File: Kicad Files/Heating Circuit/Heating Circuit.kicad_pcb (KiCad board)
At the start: 2 copper layers, 73 x 78 mm, 12 parts, among them J1 XT60_F_16.6V, J2 XT60_F_Heater, J3 XT60_F_Thermocouple, Q1 BUK9M52-40EX, U1 MAX31855KASA+T

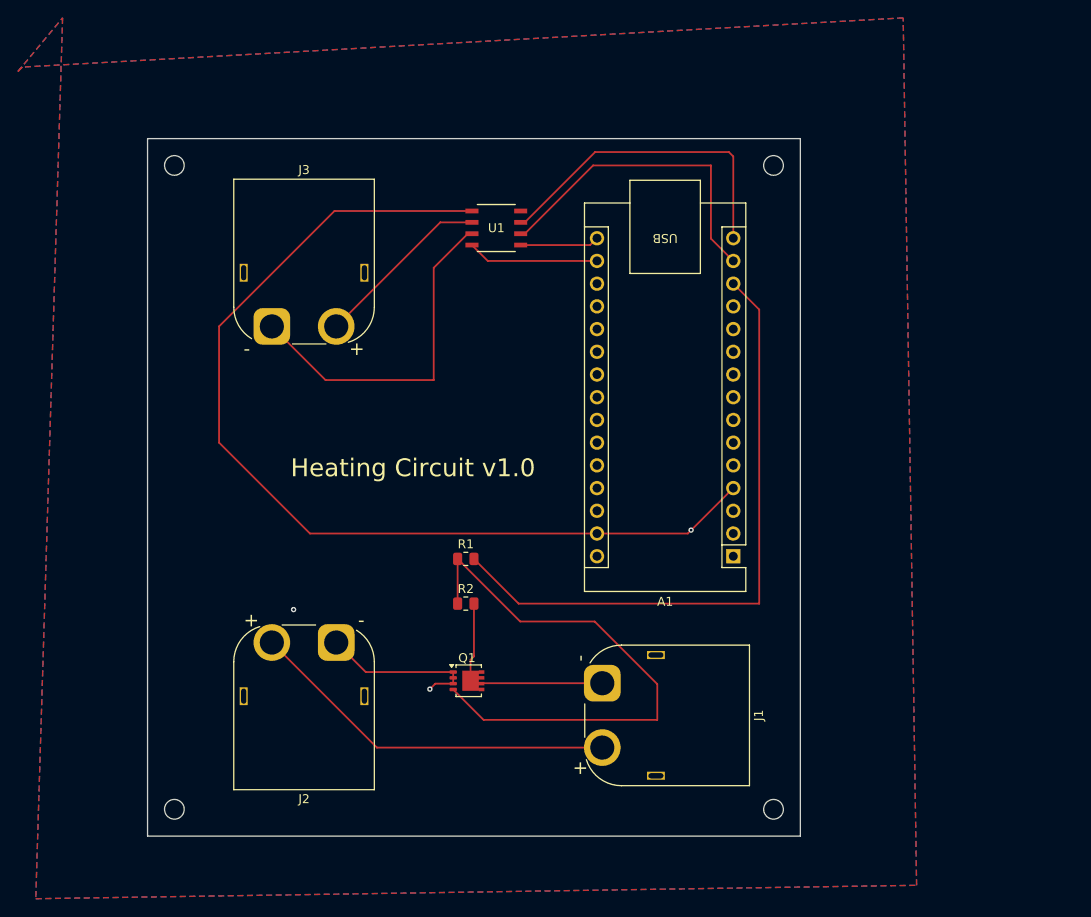
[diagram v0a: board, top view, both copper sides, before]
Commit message: Fixed PWM direction, rerouted PCB trades
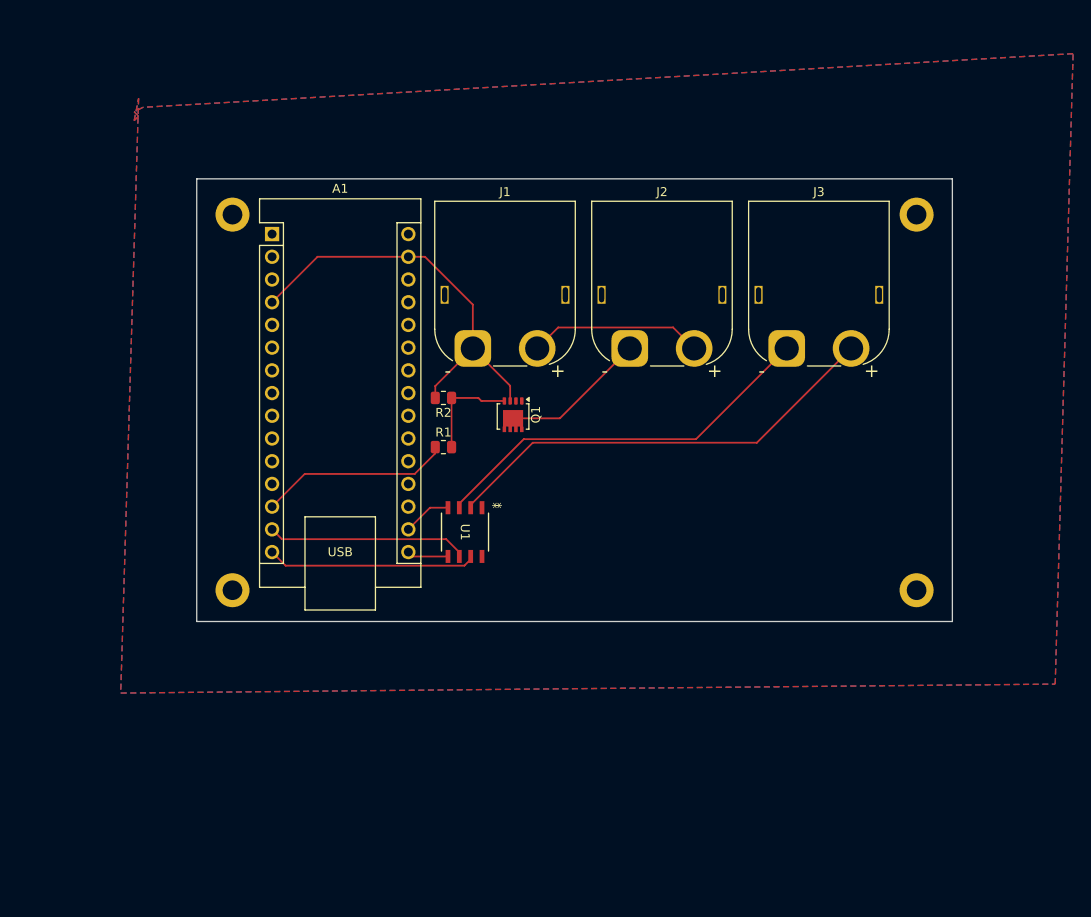
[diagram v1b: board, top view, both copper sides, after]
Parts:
- removed the REF** at (154.0, 104.0)
- removed the REF** at (154.0, 176.0)
- removed the REF** at (87.0, 176.0)
- removed the REF** at (87.0, 104.0)
- added REF**: MountingHole_2.2mm_M2_DIN965_Pad, MountingHole:MountingHole_2.2mm_M2_DIN965_Pad, F.Cu at (170.0, 151.5)
- added REF**: MountingHole_2.2mm_M2_DIN965_Pad, MountingHole:MountingHole_2.2mm_M2_DIN965_Pad, F.Cu at (170.0, 109.5)
- added REF**: MountingHole_2.2mm_M2_DIN965_Pad, MountingHole:MountingHole_2.2mm_M2_DIN965_Pad, F.Cu at (93.5, 109.5)
- added REF**: MountingHole_2.2mm_M2_DIN965_Pad, MountingHole:MountingHole_2.2mm_M2_DIN965_Pad, F.Cu at (93.5, 151.5)
- moved A1 62.9 mm to (97.9, 111.7), turned to 0 degrees
- moved J3 57.6 mm to (155.5, 124.5)
- moved J2 46.5 mm to (137.9, 124.5), turned to 0 degrees
- moved J1 40.1 mm to (120.4, 124.5), turned to 0 degrees
- moved U1 34.2 mm to (119.5, 145.0), turned to -90 degrees
- moved Q1 30.2 mm to (124.9, 131.9), turned to -90 degrees
- moved R2 23.1 mm to (117.1, 130.0), turned to 180 degrees
- moved R1 12.7 mm to (117.1, 135.5)
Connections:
- net VCC_heater renamed +16.4V
- J1 pad 1: Net-(J1-Pin_1) -> GND_16.4V
- Q1 pad 5: Net-(J1-Pin_1) -> GND_16.4V
- R1 pad 1: Net-(Q1-G) -> PWM_heater
- R1 pad 2: PWM_heater -> Net-(Q1-G)
- R2 pad 2: Net-(J1-Pin_1) -> GND_16.4V
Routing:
- net GND_16.4V: track 129.1 -> 62.8 mm, vias 3 -> 0
- net Net-(Q1-G): track 61.4 -> 11.5 mm
- net PWM_heater: track 71.0 -> 21.4 mm
- net Net-(J3-Pin_2): track 20.0 -> 50.1 mm
- net Net-(J1-Pin_1): track 23.6 -> 0.00 mm
- net +16.4V: track 41.8 -> 19.5 mm
- net CS_thermocouple: track 36.2 -> 22.5 mm
- net MISO_thermocouple: track 36.4 -> 23.5 mm
- net 3.3V_ard: track 14.7 -> 5.43 mm
- net Net-(J3-Pin_1): track 39.0 -> 44.3 mm
- net CLK: track 8.85 -> 4.63 mm
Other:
- board size 73 x 78 mm -> 84.5 x 49.5 mm
- board text removed: "Heating Circuit v1.0"
